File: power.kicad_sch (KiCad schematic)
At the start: 18 parts, among them J1 Barrel_Jack, U12 AMS1117-3.3, U3 AMS1117-ADJ, U5 TLV74010PDQNR

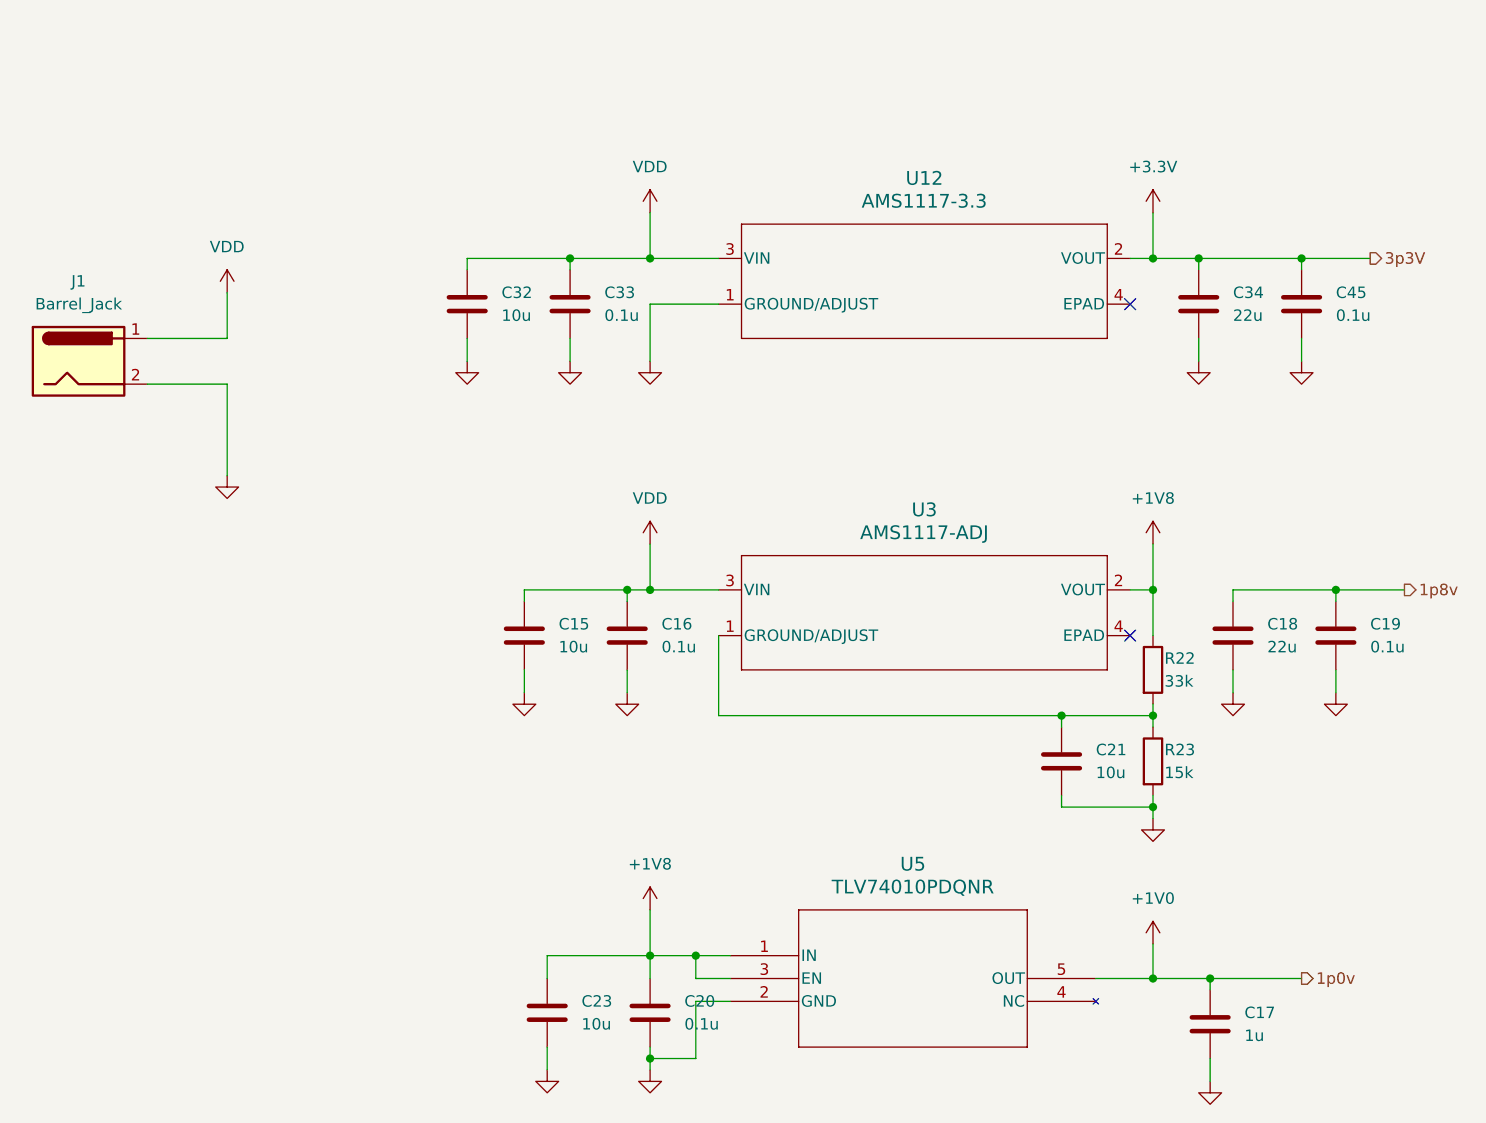
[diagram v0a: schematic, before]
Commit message: Finalized schematic
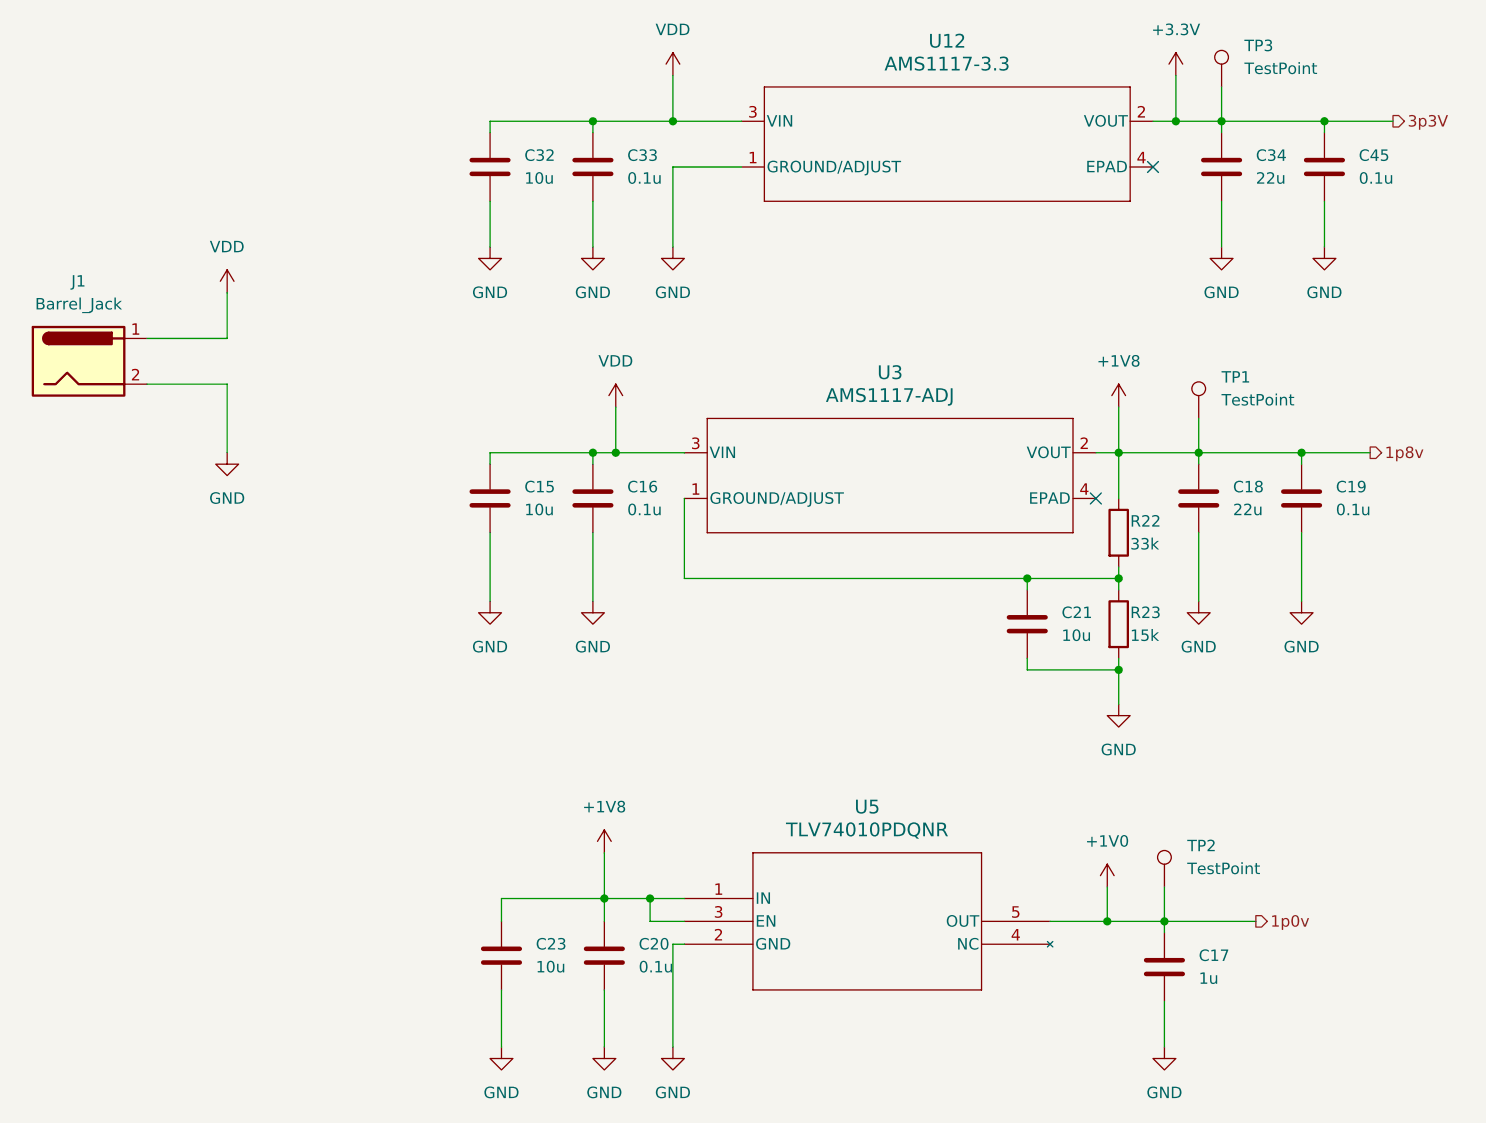
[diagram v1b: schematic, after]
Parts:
- added TP1, TP2, TP3: TestPoint, TestPoint:TestPoint_Pad_1.5x1.5mm, symbol Connector:TestPoint
- C15, C16, C17, C18, C19, C20, C21, C23, C32, C33, C34, C45: footprint (none) -> Capacitor_SMD:C_0402_1005Metric
- J1: footprint (none) -> Connector_BarrelJack:BarrelJack_Horizontal
- R22, R23: footprint (none) -> Resistor_SMD:R_0402_1005Metric
- U12: footprint SOT_AMS_ADS -> TeenieWeenieLibrary:SOT_AMS_ADS
- U3: footprint SOT_AMS_ADS -> Connector_BarrelJack:BarrelJack_Horizontal
- U5: footprint SOT_PDQNR_TEX -> TeenieWeenieLibrary:SOT_PDQNR_TEX
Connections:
- net 1p8v is gone; now on net +1V8: C18.1, C19.1
- net +1V0: now also TP2.1
- net +1V8: now also TP1.1
- net +3.3V: now also TP3.1
- net GNDA renamed GND
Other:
- moved on the sheet: C15, C16, C17, C18, C19, C20, C21, C23, C32, C33, C34, C45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
